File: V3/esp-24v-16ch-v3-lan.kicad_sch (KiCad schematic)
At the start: 19 parts, among them J7 ETHERNET, U5 LAN8710A

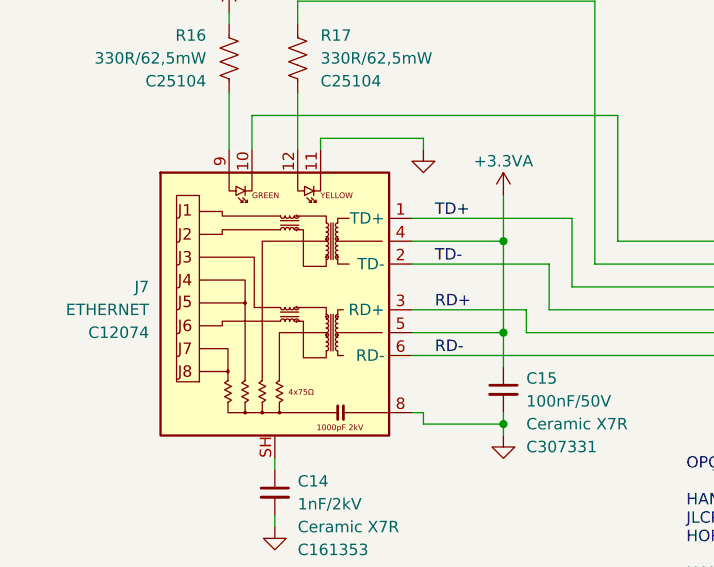
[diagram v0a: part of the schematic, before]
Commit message: Adjusted version numbers
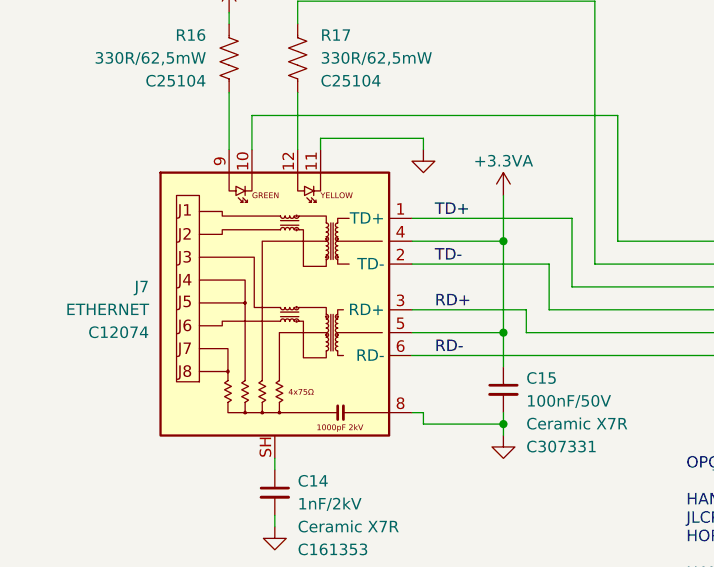
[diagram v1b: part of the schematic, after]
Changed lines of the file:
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@@
 (kicad_sch
-	(version 20231120)
+	(version 20250114)
 	(generator "eeschema")
-	(generator_version "8.0")
+	(generator_version "9.0")
 	(paper "A4")
 	(title_block
@@
 		(rev "V3.2")
 	)
+	(text "OPÇÕES RJ45\n\nHANRUN HR911105A\nJLCPCB C12074\nHORIZONTAL MAGNÉTICO\n\nHANRUN HY951180A\nJLCPCB C34677\nVERTICAL MAGNÉTICO"
+		(exclude_from_sim no)
+		(at 93.98 191.77 0)
+		(effects
+			(font
+				(size 1.27 1.27)
+			)
+			(justify left bottom)
+		)
+	)
 	(junction
 		(at 67.31 31.75)
@@
 		)
 	)
-	(text "OPÇÕES RJ45\n\nHANRUN HR911105A\nJLCPCB C12074\nHORIZONTAL MAGNÉTICO\n\nHANRUN HY951180A\nJLCPCB C34677\nVERTICAL MAGNÉTICO"
-		(exclude_from_sim no)
-		(at 93.98 191.77 0)
-		(effects
-			(font
-				(size 1.27 1.27)
-			)
-			(justify left bottom)
-		)
-	)
 	(label "RD-"
 		(at 66.04 162.56 0)
-		(fields_autoplaced yes)
 		(effects
 			(font
@@
 	(label "LED_Y_A"
 		(at 199.39 81.28 0)
-		(fields_autoplaced yes)
 		(effects
 			(font
@@
 	(label "TD+"
 		(at 66.04 147.32 0)
-		(fields_autoplaced yes)
 		(effects
 			(font
@@
 	(label "TD+"
 		(at 199.39 60.96 0)
-		(fields_autoplaced yes)
 		(effects
 			(font
@@
 	(label "TD-"
 		(at 66.04 152.4 0)
-		(fields_autoplaced yes)
 		(effects
 			(font
@@
 	(label "RD-"
 		(at 199.39 68.58 0)
-		(fields_autoplaced yes)
 		(effects
 			(font
@@
 	(label "RD+"
 		(at 66.04 157.48 0)
-		(fields_autoplaced yes)
 		(effects
 			(font
@@
 	(label "RD+"
 		(at 199.39 66.04 0)
-		(fields_autoplaced yes)
 		(effects
 			(font
@@
 	(label "LED_G_K"
 		(at 199.39 83.82 0)
-		(fields_autoplaced yes)
 		(effects
 			(font
@@
 	(label "TD-"
 		(at 199.39 63.5 0)
-		(fields_autoplaced yes)
 		(effects
 			(font
@@
 		(shape output)
 		(at 34.29 73.66 180)
-		(fields_autoplaced yes)
 		(effects
 			(font
@@
 		(shape output)
 		(at 34.29 68.58 180)
-		(fields_autoplaced yes)
 		(effects
 			(font
@@
 		(shape input)
 		(at 34.29 109.22 180)
-		(fields_autoplaced yes)
 		(effects
 			(font
@@
 		(shape input)
 		(at 34.29 78.74 180)
-		(fields_autoplaced yes)
 		(effects
 			(font
@@
 		(shape output)
 		(at 34.29 106.68 180)
-		(fields_autoplaced yes)
 		(effects
 			(font
@@
 		(shape input)
 		(at 34.29 76.2 180)
-		(fields_autoplaced yes)
 		(effects
 			(font
@@
 		(shape input)
 		(at 34.29 71.12 180)
-		(fields_autoplaced yes)
 		(effects
 			(font
@@
 		(shape output)
 		(at 34.29 58.42 180)
-		(fields_autoplaced yes)
 		(effects
 			(font
@@
 		(shape output)
 		(at 34.29 60.96 180)
-		(fields_autoplaced yes)
 		(effects
 			(font
@@
 		)
 	)
+	(embedded_fonts no)
 )
